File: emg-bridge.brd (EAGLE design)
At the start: 91.5 x 50.8 mm, 29 parts, among them J1 RJ25_4X1, J2 RJ25_4X1, J3 M03_0.156IN-RA, J4 POWER_JACKPTH, J5 USB-B, J6 M05X2RAF, U1 DC_ISOLATOR-RKZ0505D

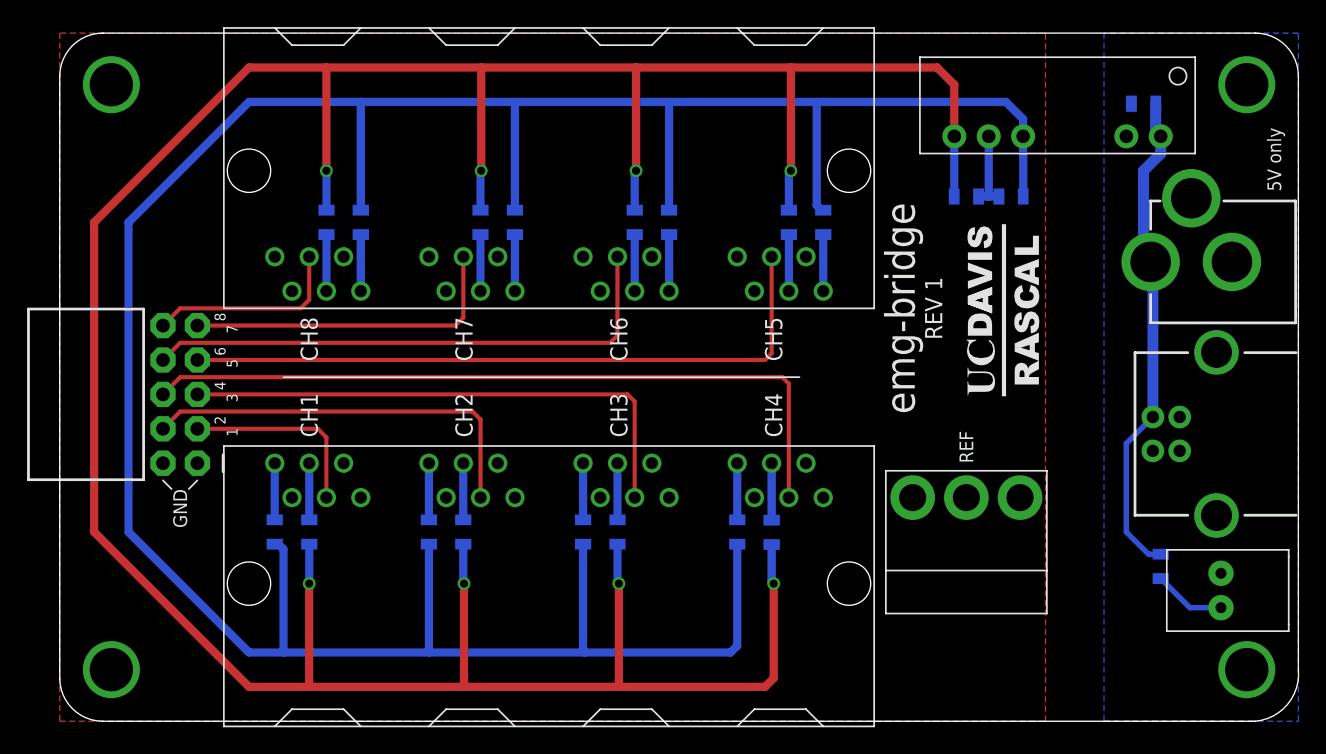
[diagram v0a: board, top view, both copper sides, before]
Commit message: Minor changes. Revision 1 should really be ready this time.
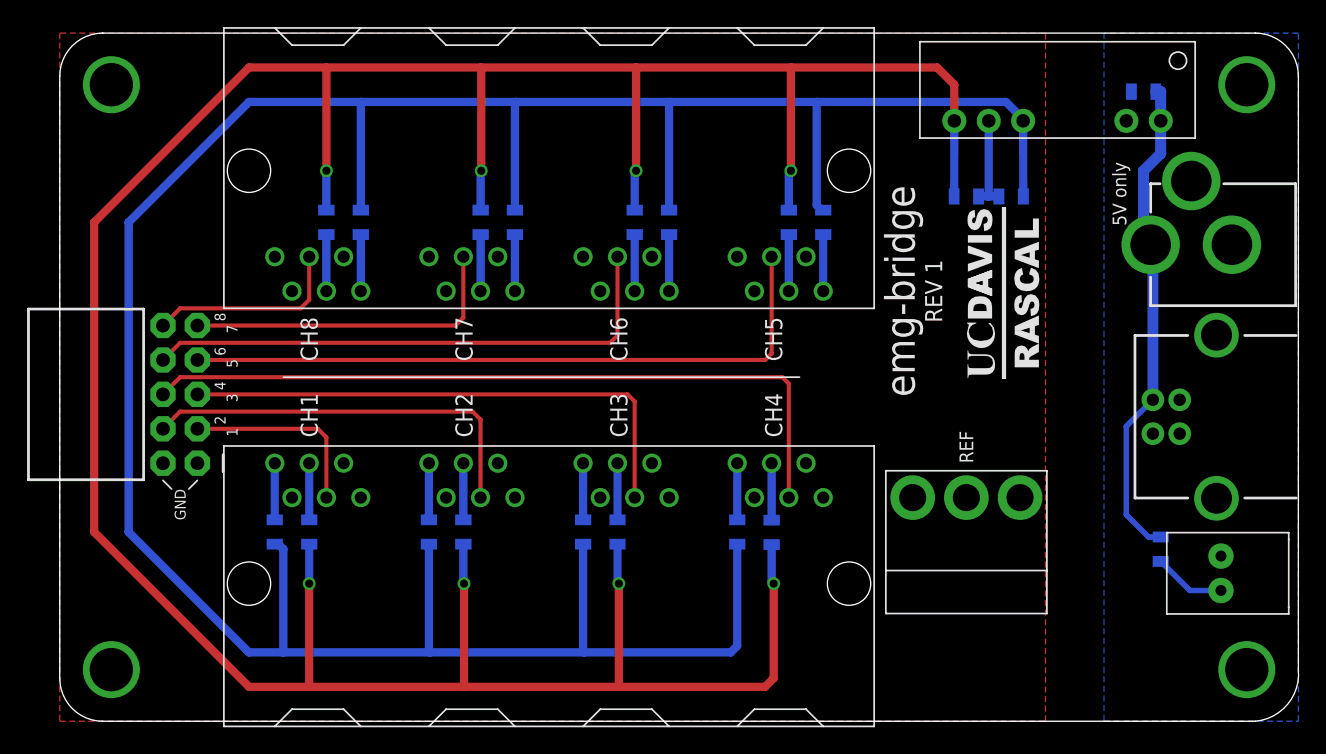
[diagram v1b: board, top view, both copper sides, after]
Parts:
- R17: value (none) -> 1k
- moved J4 1.27 mm to (94.2, 35.2)
- moved D1 1.27 mm to (85.7, 10.9)
- moved J5 1.27 mm to (82.7, 22.5)
- moved R17 1.27 mm to (81.3, 12.7)
- moved U$1 1.27 mm to (69.7, 31.6)
- moved U1 1.14 mm to (81.3, 44.3)
- moved C1 0.89 mm to (80.0, 46.5)
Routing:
- net GND: track 5.95 -> 7.09 mm
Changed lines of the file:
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@@
 <wire x1="3.175" y1="50.8" x2="0" y2="47.625" width="0" layer="20" curve="90"/>
 <wire x1="88.265" y1="50.8" x2="91.44" y2="47.625" width="0" layer="20" curve="-90"/>
-<text x="63.119" y="30.48" size="2.1844" layer="21" font="vector" ratio="15" rot="R90" align="bottom-center">emg-bridge</text>
-<text x="65.151" y="30.48" size="1.27" layer="21" font="vector" ratio="10" rot="R90" align="bottom-center">REV 1</text>
+<text x="63.119" y="31.75" size="2.1844" layer="21" font="vector" ratio="15" rot="R90" align="bottom-center">emg-bridge</text>
+<text x="65.151" y="31.75" size="1.27" layer="21" font="vector" ratio="10" rot="R90" align="bottom-center">REV 1</text>
 <text x="18.415" y="20.955" size="1.27" layer="21" font="vector" ratio="12" rot="R90" align="center-left">CH1</text>
 <text x="29.845" y="20.955" size="1.27" layer="21" font="vector" ratio="12" rot="R90" align="center-left">CH2</text>
@@
 <text x="12.319" y="26.416" size="0.8128" layer="21" font="vector" ratio="10" rot="R90" align="top-center">5</text>
 <text x="12.319" y="28.956" size="0.8128" layer="21" font="vector" ratio="10" rot="R90" align="top-center">7</text>
-<text x="8.89" y="17.145" size="1.016" layer="21" font="vector" ratio="10" rot="R90" align="center-right">GND</text>
+<text x="8.89" y="17.145" size="0.8128" layer="21" font="vector" ratio="10" rot="R90" align="center-right">GND</text>
 <wire x1="8.255" y1="17.145" x2="7.62" y2="17.78" width="0.127" layer="21"/>
 <wire x1="9.525" y1="17.145" x2="10.16" y2="17.78" width="0.127" layer="21"/>
@@
 <text x="11.43" y="27.305" size="0.8128" layer="21" font="vector" ratio="10" rot="R90" align="top-center">6</text>
 <text x="11.43" y="29.845" size="0.8128" layer="21" font="vector" ratio="10" rot="R90" align="top-center">8</text>
-<text x="90.17" y="39.116" size="1.016" layer="21" font="vector" ratio="10" rot="R90">5V only</text>
+<text x="78.74" y="36.576" size="1.016" layer="21" font="vector" ratio="10" rot="R90">5V only</text>
 </plain>
 <attributes>
@@
 <element name="J3" library="eagle-lib" package="TE_640389-3" value="M03_0.156IN-RA" x="66.929" y="16.51" smashed="yes" rot="R180"/>
 <element name="J6" library="SparkFun-Connectors" package="2X5-RAF" value="M05X2RAF" x="8.89" y="24.13" smashed="yes" rot="R180"/>
-<element name="U$1" library="ucdrascal-eagle-lib" package="UCDAVIS-RASCAL_LOGO" value="UCDAVIS-RASCAL_LOGO-2LINE" x="69.723" y="30.353" rot="R90"/>
-<element name="U1" library="eagle-lib" package="SIP7" value="DC_ISOLATOR-RKZ0505D" x="81.28" y="43.18" rot="R180"/>
-<element name="J5" library="SparkFun-Connectors" package="USB-B-PTH" value="USB-B" x="82.677" y="21.209" smashed="yes" rot="R180">
-<attribute name="PROD_ID" value="CONN-08278" x="82.677" y="21.209" size="1.778" layer="27" rot="R180" display="off"/>
-</element>
-<element name="C1" library="SparkFun-Capacitors" package="0805" value="0.1uF" x="80.01" y="45.593" smashed="yes" rot="MR0">
-<attribute name="NAME" x="80.01" y="46.5455" size="0.4064" layer="26" font="vector" rot="MR180" align="top-center"/>
+<element name="U$1" library="ucdrascal-eagle-lib" package="UCDAVIS-RASCAL_LOGO" value="UCDAVIS-RASCAL_LOGO-2LINE" x="69.723" y="31.623" rot="R90"/>
+<element name="U1" library="eagle-lib" package="SIP7" value="DC_ISOLATOR-RKZ0505D" x="81.28" y="44.323" rot="R180"/>
+<element name="J5" library="SparkFun-Connectors" package="USB-B-PTH" value="USB-B" x="82.677" y="22.479" smashed="yes" rot="R180">
+<attribute name="PROD_ID" value="CONN-08278" x="82.677" y="22.479" size="1.778" layer="27" rot="R180" display="off"/>
+</element>
+<element name="C1" library="SparkFun-Capacitors" package="0805" value="0.1uF" x="80.01" y="46.482" smashed="yes" rot="MR0">
+<attribute name="NAME" x="80.01" y="47.4345" size="0.4064" layer="26" font="vector" rot="MR180" align="top-center"/>
 </element>
 <element name="C2" library="SparkFun-Capacitors" package="0805" value="0.1uF" x="66.929" y="38.735" smashed="yes" rot="MR180">
@@
 <attribute name="NAME" x="70.231" y="37.6555" size="0.4064" layer="26" font="vector" rot="MR0" align="top-center"/>
 </element>
-<element name="J4" library="SparkFun-Connectors" package="POWER_JACK_PTH" value="POWER_JACKPTH" x="94.234" y="33.909" smashed="yes" rot="R90"/>
-<element name="D1" library="eagle-lib" package="LED_RA" value="LED_LA93B" x="85.725" y="9.652" smashed="yes" rot="R90"/>
-<element name="R17" library="SparkFun-Passives" package="0805" value="" x="81.28" y="11.43" smashed="yes" rot="MR90">
-<attribute name="NAME" x="80.137" y="11.3665" size="0.4064" layer="26" font="vector" rot="MR0"/>
-<attribute name="VALUE" x="79.883" y="10.414" size="0.4064" layer="28" rot="MR90"/>
+<element name="J4" library="SparkFun-Connectors" package="POWER_JACK_PTH" value="POWER_JACKPTH" x="94.234" y="35.179" smashed="yes" rot="R90"/>
+<element name="D1" library="eagle-lib" package="LED_RA" value="LED_LA93B" x="85.725" y="10.922" smashed="yes" rot="R90"/>
+<element name="R17" library="SparkFun-Passives" package="0805" value="1k" x="81.28" y="12.7" smashed="yes" rot="MR90">
+<attribute name="NAME" x="80.137" y="12.6365" size="0.4064" layer="26" font="vector" rot="MR0"/>
 </element>
 </elements>
@@
 <contactref element="C2" pad="2"/>
 <contactref element="C3" pad="1"/>
-<wire x1="68.58" y1="43.18" x2="68.58" y2="38.735" width="0.6096" layer="16"/>
+<wire x1="68.58" y1="44.323" x2="68.58" y2="38.735" width="0.6096" layer="16"/>
 <wire x1="69.331" y1="38.735" x2="68.58" y2="38.735" width="0.6096" layer="16"/>
 <wire x1="67.829" y1="38.735" x2="68.58" y2="38.735" width="0.6096" layer="16"/>
@@
 <contactref element="R15" pad="2"/>
 <contactref element="U1" pad="7"/>
-<wire x1="66.04" y1="43.18" x2="66.04" y2="46.99" width="0.6096" layer="1"/>
+<wire x1="66.04" y1="44.323" x2="66.04" y2="46.99" width="0.6096" layer="1"/>
 <wire x1="66.04" y1="46.99" x2="64.77" y2="48.26" width="0.6096" layer="1"/>
 <wire x1="64.77" y1="48.26" x2="53.975" y2="48.26" width="0.6096" layer="1"/>
@@
 <wire x1="53.975" y1="40.64" x2="53.975" y2="48.26" width="0.6096" layer="1"/>
 <contactref element="C2" pad="1"/>
-<wire x1="66.029" y1="38.735" x2="66.04" y2="43.18" width="0.6096" layer="16"/>
+<wire x1="66.029" y1="38.735" x2="66.04" y2="44.323" width="0.6096" layer="16"/>
 </signal>
 <signal name="-VE">
@@
 <contactref element="R16" pad="2"/>
 <contactref element="U1" pad="5"/>
-<wire x1="71.12" y1="43.18" x2="71.12" y2="44.45" width="0.6096" layer="16"/>
+<wire x1="71.12" y1="44.323" x2="71.12" y2="44.45" width="0.6096" layer="16"/>
 <wire x1="71.12" y1="44.45" x2="69.85" y2="45.72" width="0.6096" layer="16"/>
 <wire x1="69.85" y1="45.72" x2="55.88" y2="45.72" width="0.6096" layer="16"/>
@@
 <wire x1="55.88" y1="38.1" x2="55.88" y2="45.72" width="0.6096" layer="16"/>
 <contactref element="C3" pad="2"/>
-<wire x1="71.131" y1="38.735" x2="71.12" y2="43.18" width="0.6096" layer="16"/>
+<wire x1="71.131" y1="38.735" x2="71.12" y2="44.323" width="0.6096" layer="16"/>
 </signal>
 <signal name="N$8">
@@
 <contactref element="J4" pad="PWR"/>
 <contactref element="J5" pad="VBUS"/>
-<wire x1="80.91" y1="45.593" x2="80.91" y2="43.55" width="0.8128" layer="16"/>
-<wire x1="80.91" y1="43.55" x2="81.28" y2="43.18" width="0.8128" layer="16"/>
-<wire x1="80.6958" y1="22.459" x2="80.6958" y2="33.7472" width="0.8128" layer="16"/>
-<wire x1="80.6958" y1="33.7472" x2="80.534" y2="33.909" width="0.8128" layer="16"/>
-<wire x1="81.28" y1="43.18" x2="81.28" y2="41.91" width="0.8128" layer="16"/>
+<wire x1="80.6958" y1="23.729" x2="80.6958" y2="35.0172" width="0.8128" layer="16"/>
+<wire x1="80.6958" y1="35.0172" x2="80.534" y2="35.179" width="0.8128" layer="16"/>
+<wire x1="81.28" y1="44.323" x2="81.28" y2="41.91" width="0.8128" layer="16"/>
 <wire x1="81.28" y1="41.91" x2="80.01" y2="40.64" width="0.8128" layer="16"/>
-<wire x1="80.01" y1="40.64" x2="80.01" y2="34.433" width="0.8128" layer="16"/>
-<wire x1="80.01" y1="34.433" x2="80.534" y2="33.909" width="0.8128" layer="16"/>
+<wire x1="80.01" y1="40.64" x2="80.01" y2="35.703" width="0.8128" layer="16"/>
+<wire x1="80.01" y1="35.703" x2="80.534" y2="35.179" width="0.8128" layer="16"/>
 <contactref element="R17" pad="2"/>
-<wire x1="81.28" y1="12.33" x2="80.38" y2="12.33" width="0.4064" layer="16"/>
-<wire x1="80.38" y1="12.33" x2="78.74" y2="13.97" width="0.4064" layer="16"/>
-<wire x1="78.74" y1="13.97" x2="78.74" y2="20.5032" width="0.4064" layer="16"/>
-<wire x1="78.74" y1="20.5032" x2="80.6958" y2="22.459" width="0.4064" layer="16"/>
+<wire x1="81.28" y1="13.6" x2="80.38" y2="13.6" width="0.4064" layer="16"/>
+<wire x1="80.38" y1="13.6" x2="78.74" y2="15.24" width="0.4064" layer="16"/>
+<wire x1="78.74" y1="15.24" x2="78.74" y2="21.7732" width="0.4064" layer="16"/>
+<wire x1="78.74" y1="21.7732" x2="80.6958" y2="23.729" width="0.4064" layer="16"/>
+<wire x1="80.91" y1="46.482" x2="81.28" y2="46.482" width="0.8128" layer="16"/>
+<wire x1="81.28" y1="46.482" x2="81.28" y2="44.323" width="0.8128" layer="16"/>
 </signal>
 <signal name="N$4">
 <contactref element="R17" pad="1"/>
 <contactref element="D1" pad="A"/>
-<wire x1="85.725" y1="8.382" x2="83.428" y2="8.382" width="0.4064" layer="16"/>
-<wire x1="83.428" y1="8.382" x2="81.28" y2="10.53" width="0.4064" layer="16"/>
+<wire x1="85.725" y1="9.652" x2="83.428" y2="9.652" width="0.4064" layer="16"/>
+<wire x1="83.428" y1="9.652" x2="81.28" y2="11.8" width="0.4064" layer="16"/>
 </signal>
 </signals>
